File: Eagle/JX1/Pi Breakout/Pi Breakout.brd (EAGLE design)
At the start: 88.9 x 55.9 mm, 4 parts, among them J2 RASPBERRYPI-40-PIN-GPIO_PTH_N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

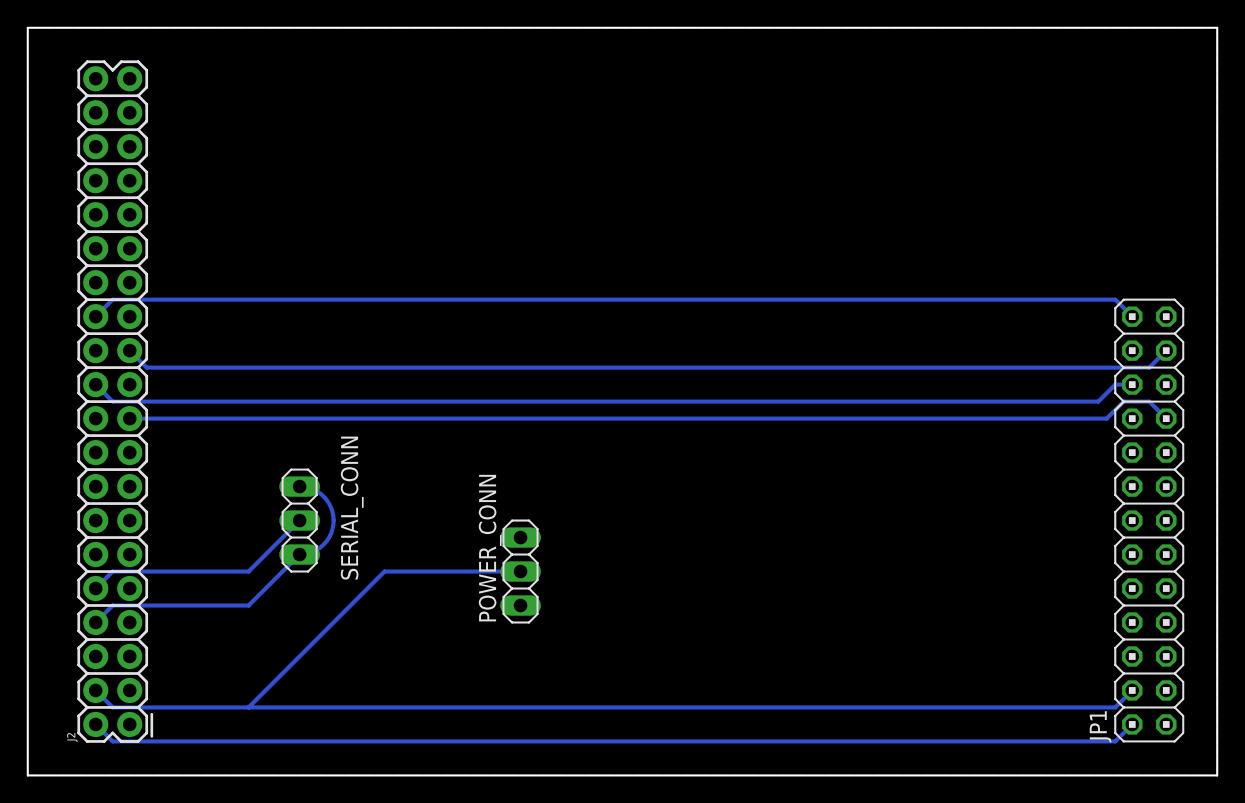
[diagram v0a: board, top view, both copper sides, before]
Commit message: Fixes to breakout
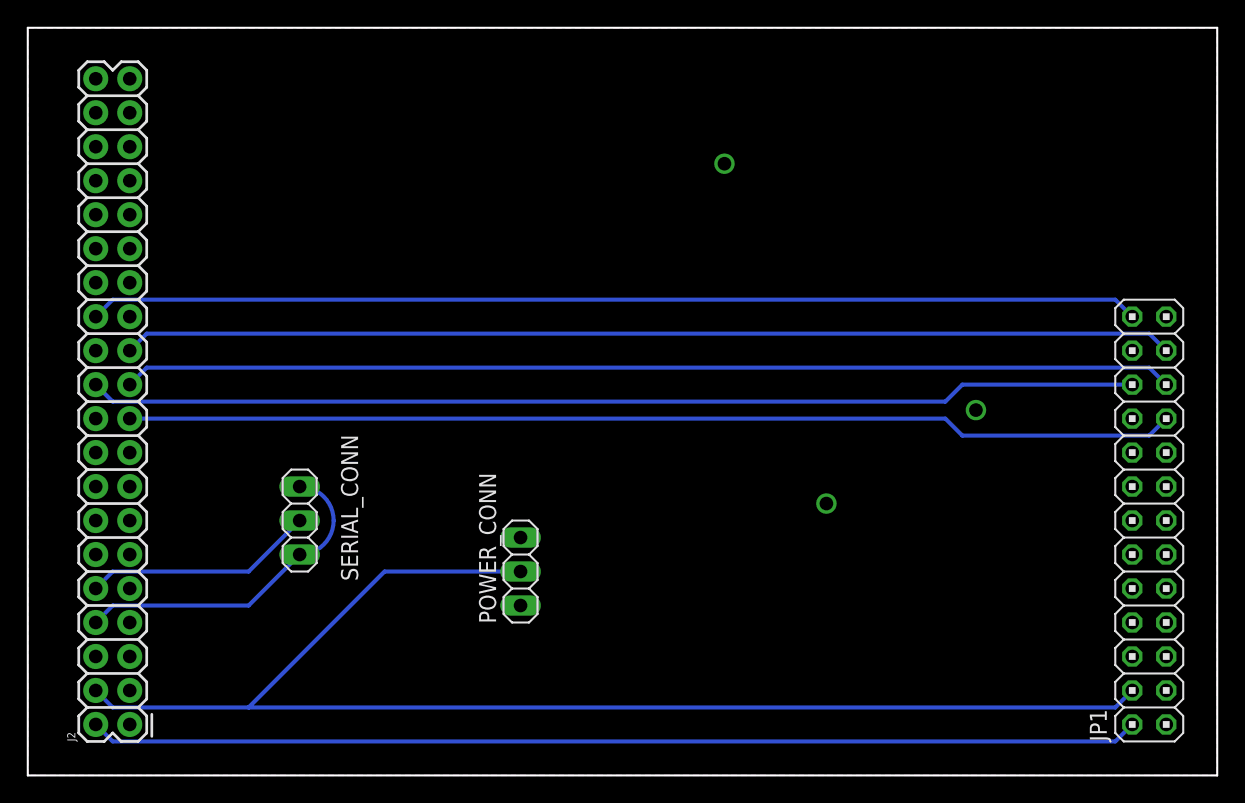
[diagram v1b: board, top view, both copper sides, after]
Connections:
- removed net GND@25: JP1.25
- removed net N$39: J2.21
- net GND: now also JP1.25
- net MISO: now also J2.21
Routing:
- net MISO: track 0.00 -> 78.5 mm
- added copper zone on layer 1, net GND
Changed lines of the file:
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@@
 </class>
 </classes>
-<designrules name="default">
+<designrules name="default *">
 <description language="de">&lt;b&gt;EAGLE Design Rules&lt;/b&gt;
 &lt;p&gt;
@@
 <param name="mdViaViaSameLayer" value="6mil"/>
 <param name="mnLayersViaInSmd" value="2"/>
-<param name="mdCopperDimension" value="40mil"/>
+<param name="mdCopperDimension" value="1mil"/>
 <param name="mdDrill" value="6mil"/>
 <param name="mdSmdStop" value="0mil"/>
@@
 <contactref element="JP1" pad="5"/>
 </signal>
-<signal name="GND@25">
-<contactref element="JP1" pad="25"/>
-</signal>
 <signal name="7">
 <contactref element="JP1" pad="7"/>
@@
 <contactref element="JP1" pad="19"/>
 <contactref element="J2" pad="19"/>
-<wire x1="7.62" y1="26.67" x2="80.645" y2="26.67" width="0.3048" layer="16"/>
-<wire x1="80.645" y1="26.67" x2="81.915" y2="27.94" width="0.3048" layer="16"/>
-<wire x1="81.915" y1="27.94" x2="83.82" y2="27.94" width="0.3048" layer="16"/>
-<wire x1="83.82" y1="27.94" x2="85.09" y2="26.67" width="0.3048" layer="16"/>
+<wire x1="7.62" y1="26.67" x2="68.58" y2="26.67" width="0.3048" layer="16"/>
+<wire x1="85.09" y1="26.67" x2="83.82" y2="25.4" width="0.3048" layer="16"/>
+<wire x1="83.82" y1="25.4" x2="69.85" y2="25.4" width="0.3048" layer="16"/>
+<wire x1="69.85" y1="25.4" x2="68.58" y2="26.67" width="0.3048" layer="16"/>
 </signal>
 <signal name="MISO">
 <contactref element="JP1" pad="21"/>
+<contactref element="J2" pad="21"/>
+<wire x1="85.09" y1="29.21" x2="83.82" y2="30.48" width="0.3048" layer="16"/>
+<wire x1="83.82" y1="30.48" x2="8.89" y2="30.48" width="0.3048" layer="16"/>
+<wire x1="8.89" y1="30.48" x2="7.62" y2="29.21" width="0.3048" layer="16"/>
 </signal>
 <signal name="IRQ">
@@
 <contactref element="J2" pad="22"/>
 <wire x1="5.08" y1="29.21" x2="6.35" y2="27.94" width="0.3048" layer="16"/>
-<wire x1="6.35" y1="27.94" x2="80.01" y2="27.94" width="0.3048" layer="16"/>
-<wire x1="81.28" y1="29.21" x2="82.55" y2="29.21" width="0.3048" layer="16"/>
-<wire x1="81.28" y1="29.21" x2="80.01" y2="27.94" width="0.3048" layer="16"/>
+<wire x1="6.35" y1="27.94" x2="68.58" y2="27.94" width="0.3048" layer="16"/>
+<wire x1="69.85" y1="29.21" x2="82.55" y2="29.21" width="0.3048" layer="16"/>
+<wire x1="69.85" y1="29.21" x2="68.58" y2="27.94" width="0.3048" layer="16"/>
 </signal>
 <signal name="SCLK">
 <contactref element="JP1" pad="23"/>
 <contactref element="J2" pad="23"/>
-<wire x1="7.62" y1="31.75" x2="8.89" y2="30.48" width="0.3048" layer="16"/>
-<wire x1="8.89" y1="30.48" x2="83.82" y2="30.48" width="0.3048" layer="16"/>
-<wire x1="83.82" y1="30.48" x2="85.09" y2="31.75" width="0.3048" layer="16"/>
+<wire x1="85.09" y1="31.75" x2="83.82" y2="33.02" width="0.3048" layer="16"/>
+<wire x1="83.82" y1="33.02" x2="8.89" y2="33.02" width="0.3048" layer="16"/>
+<wire x1="7.62" y1="31.75" x2="8.89" y2="33.02" width="0.3048" layer="16"/>
 </signal>
 <signal name="24">
@@
 <contactref element="J2" pad="24"/>
 </signal>
-<signal name="N$39">
-<contactref element="J2" pad="21"/>
-</signal>
 <signal name="N$1">
 <contactref element="J2" pad="8"/>
@@
 </signal>
 <signal name="GND">
-<polygon width="0.1524" layer="16" isolate="0.6096" orphans="yes">
+<polygon width="0.1524" layer="16" isolate="0.6096">
 <vertex x="0" y="55.88"/>
 <vertex x="88.9" y="55.88"/>
@@
 <contactref element="JP1" pad="14"/>
 <contactref element="JP1" pad="20"/>
-<wire x1="7.62" y1="34.29" x2="5.08" y2="39.37" width="0" layer="19" extent="1-1"/>
-<wire x1="7.62" y1="13.97" x2="5.08" y2="8.89" width="0" layer="19" extent="1-1"/>
-<wire x1="82.55" y1="8.89" x2="85.09" y2="13.97" width="0" layer="19" extent="1-1"/>
+<contactref element="JP1" pad="25"/>
+<via x="70.866" y="27.305" extent="1-16" drill="1.02"/>
+<via x="59.69" y="20.32" extent="1-16" drill="1.02"/>
+<via x="52.07" y="45.72" extent="1-16" drill="1.02"/>
+<polygon width="0.3048" layer="1" isolate="0.4064">
+<vertex x="0" y="0"/>
+<vertex x="0" y="55.88"/>
+<vertex x="88.9" y="55.88"/>
+<vertex x="88.9" y="0"/>
+</polygon>
 </signal>
 </signals>
